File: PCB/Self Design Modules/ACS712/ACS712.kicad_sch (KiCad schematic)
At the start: 1 part, among them U1 ACS712xLCTR-20A

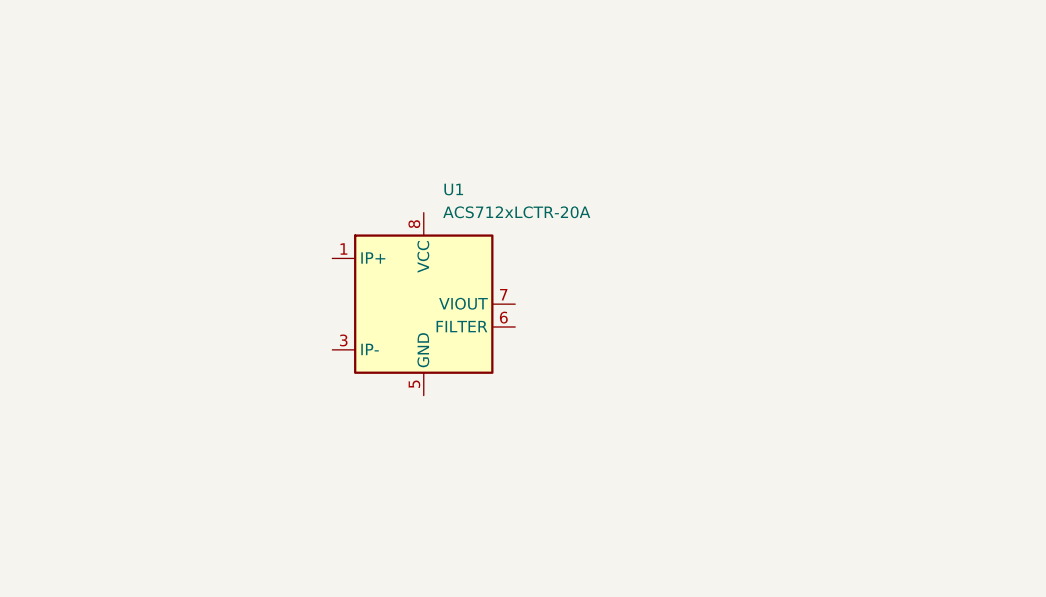
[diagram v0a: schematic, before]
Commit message: Changes Part 1 for the PCB Files
Most recent update for the PCB Design
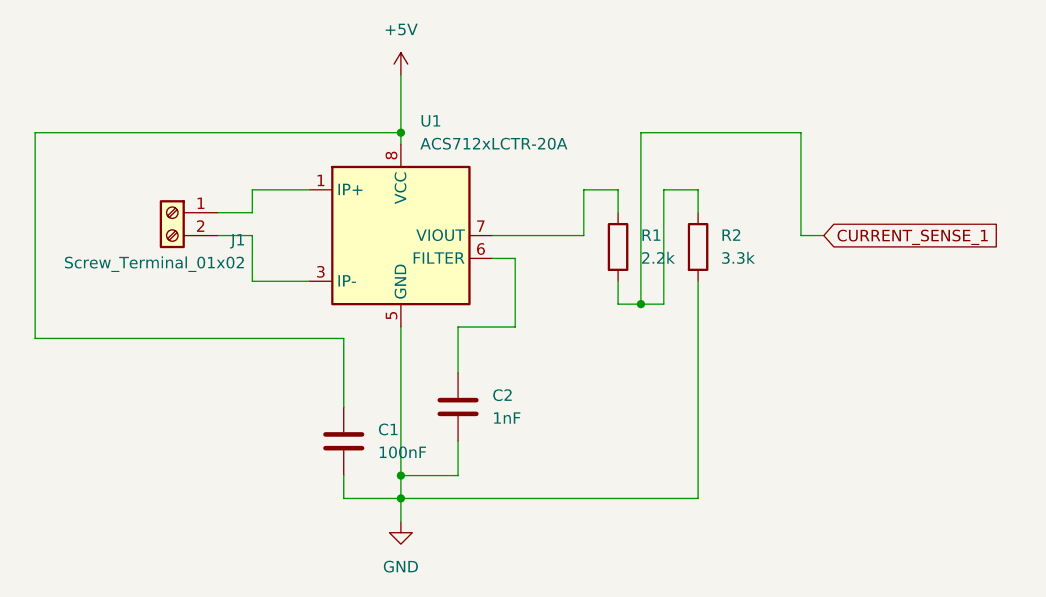
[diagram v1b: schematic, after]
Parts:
- added C1: 100nF, Capacitor_SMD:C_0805_2012Metric, symbol Device:C
- added C2: 1nF, Capacitor_SMD:C_0805_2012Metric, symbol Device:C
- added J1: Screw_Terminal_01x02, TerminalBlock_Phoenix:TerminalBlock_Phoenix_MKDS-1,5-2-5.08_1x02_P5.08mm_Horizontal, symbol Connector:Screw_Terminal_01x02
- added R1: 2.2k, Resistor_SMD:R_0805_2012Metric, symbol Device:R
- added R2: 3.3k, Resistor_SMD:R_0805_2012Metric, symbol Device:R
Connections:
- net at U1.1 (IP+), U1.2 (IP+): now also J1.1 (Pin_1)
- net at U1.3 (IP-), U1.4 (IP-): now also J1.2 (Pin_2)
- net GND: now reaches U1.5 (GND)
- net GND: now also C1.2, C2.2, R2.2
- net at U1.6 (FILTER): now also C2.1
- net at U1.7 (VIOUT): now also R1.1
- net +5V: now reaches U1.8 (VCC)
- net +5V: now also C1.1
- new net CURRENT_SENSE_1: R1.2, R2.1
